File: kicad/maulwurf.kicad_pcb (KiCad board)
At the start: 2 copper layers, 63.5 x 70 mm, 17 parts

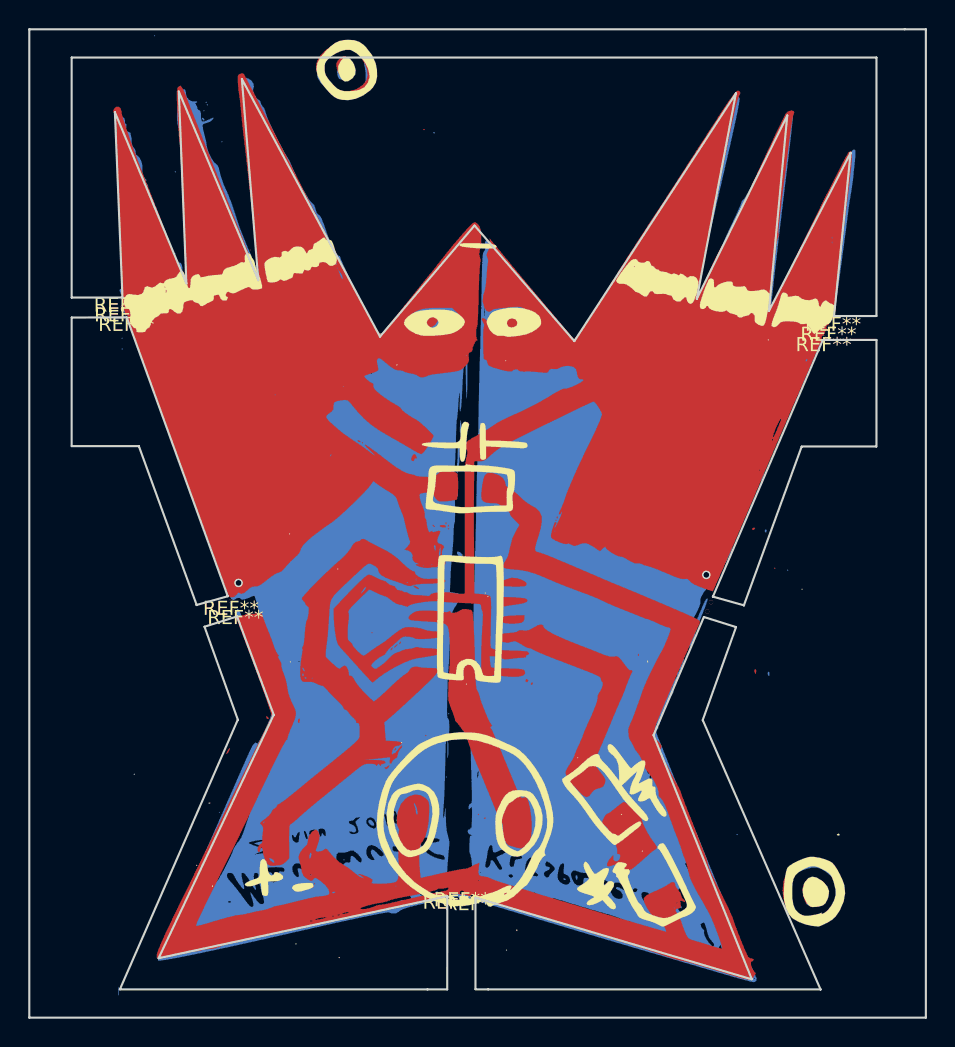
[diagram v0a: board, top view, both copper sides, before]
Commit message: Remove frame
fixes #3
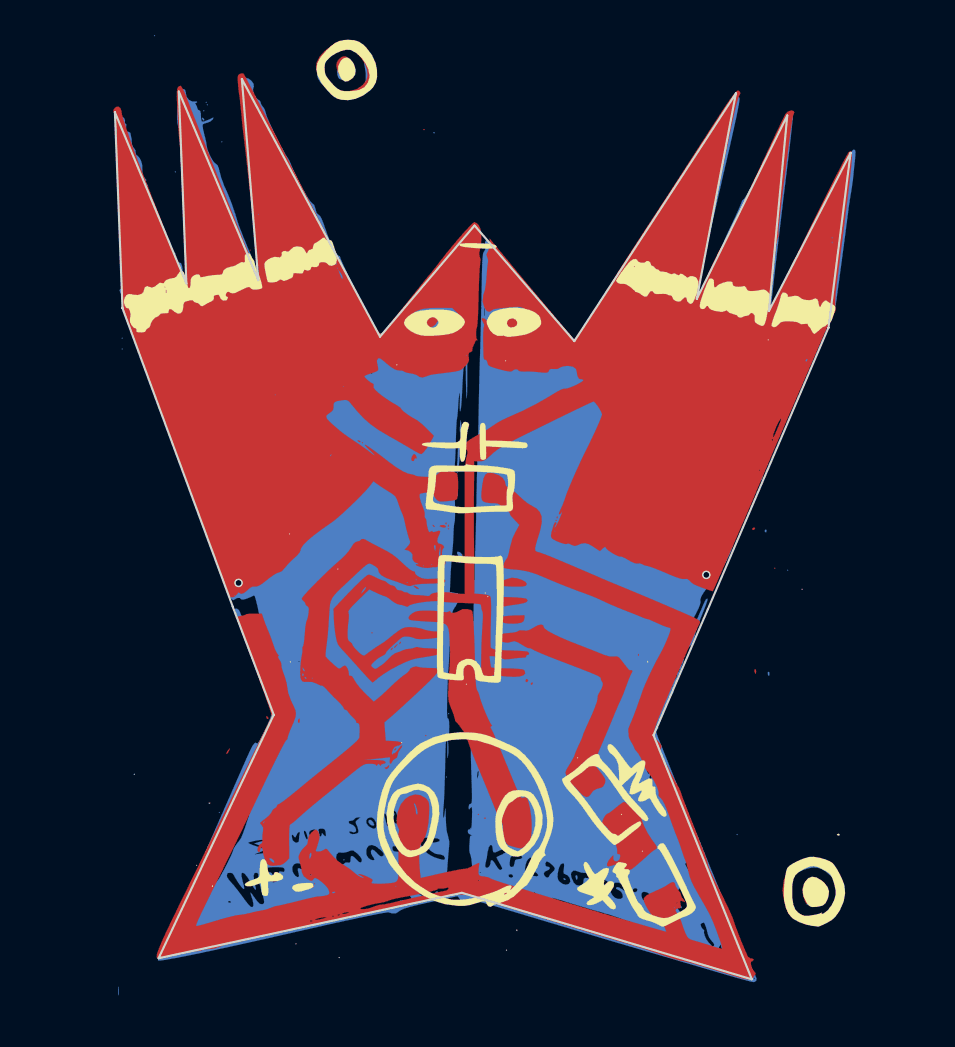
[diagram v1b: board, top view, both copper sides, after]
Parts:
- removed REF** (x13): hole, footprints:hole
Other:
- board size 63.5 x 70 mm -> 52.1 x 63.8 mm
